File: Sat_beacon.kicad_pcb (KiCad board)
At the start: 2 copper layers, 79.5 x 122.9 mm, 126 parts, among them IC1 LMX2581ESQE_NOPB, IC2 LMX2581ESQE_NOPB, J1 Conn_01x05_Pin, J2 Conn_01x03_Pin, J4 MMCX, J5 MMCX, J6 Conn_01x04_Pin, Q1 BC817-40, Q2 BC817-40, Q3 BC817-40, Q4 BC817-40, SW1 B1407, SW2 SW_Omron_B3FS, SW3 SW_Omron_B3FS, SW4 SW_Omron_B3FS, SW5 SW_Omron_B3FS, U1 LD1117DT33, U2 LD1117DT33, U3 LD1117DT33, U4 1720BL15B0050002E, U5 1720BL15B0050002E, U7 STM32C031C6Tx, Y1 FT2MHUPM10.0-T1

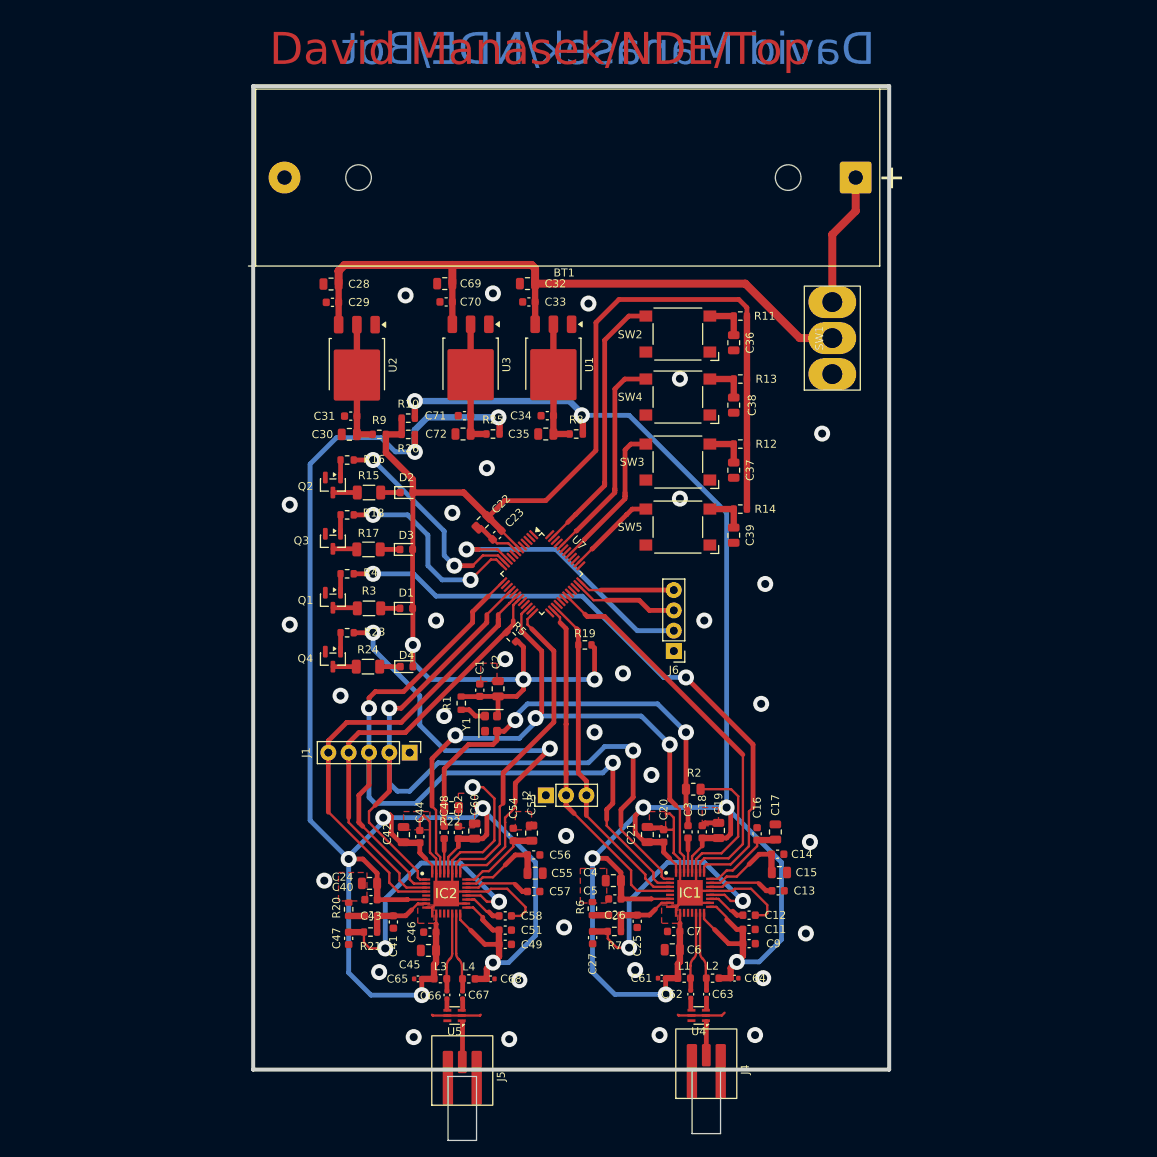
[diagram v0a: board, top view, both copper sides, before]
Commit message: PCB RF section improvement
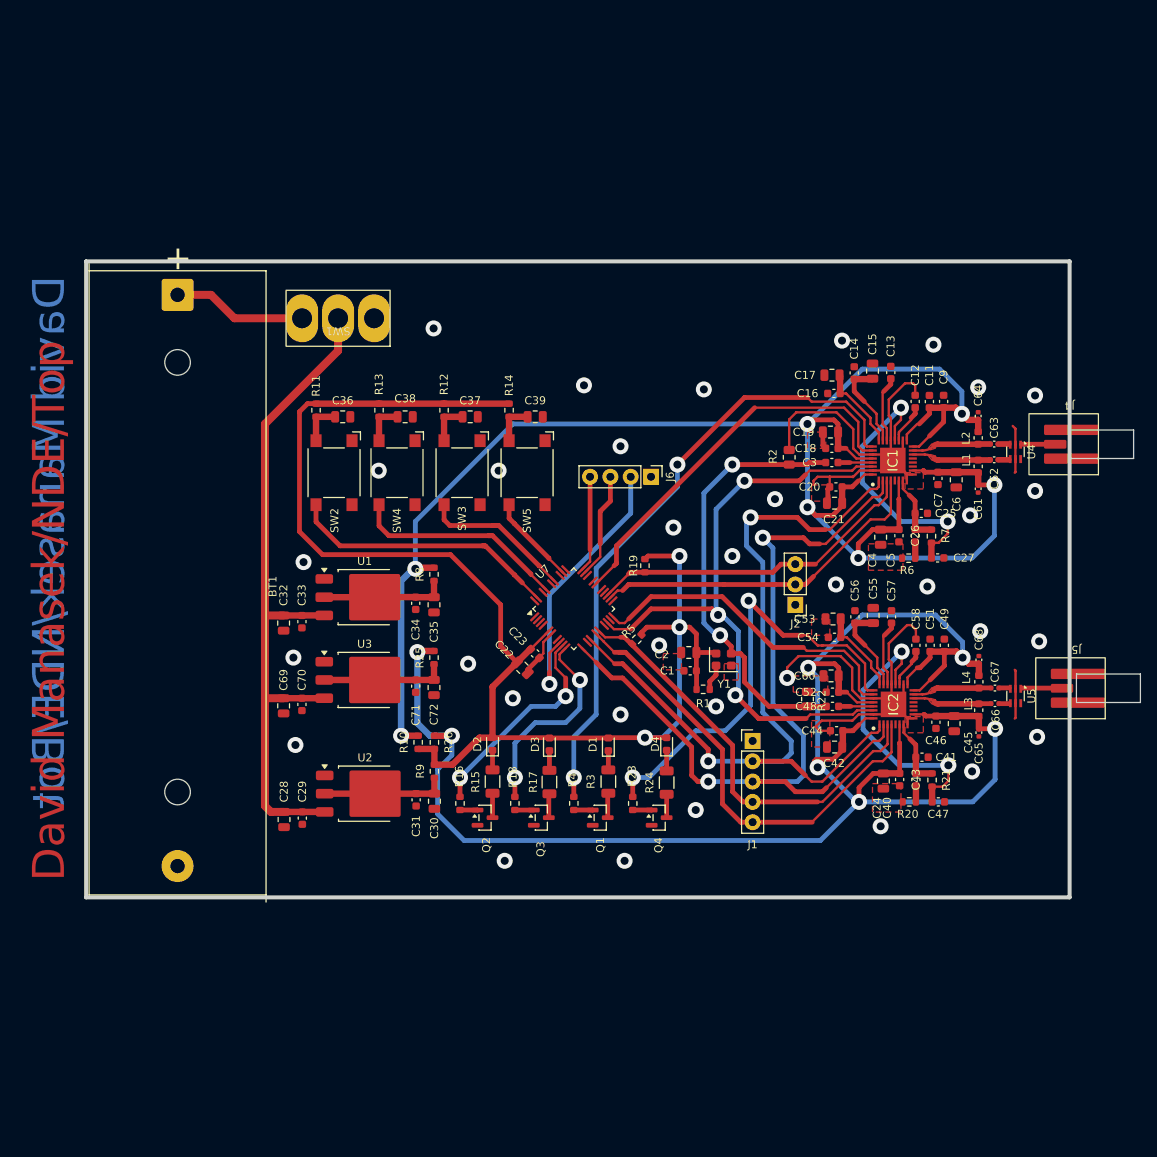
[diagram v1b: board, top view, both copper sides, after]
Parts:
- moved J5 90.8 mm to (169.2, 104.7), turned to 180 degrees
- moved J4 90.4 mm to (168.3, 74.2), turned to 180 degrees
- moved BT1 86.0 mm to (56.8, 55.6), turned to -90 degrees
- moved U4 80.8 mm to (161.6, 75.2), turned to -90 degrees
- moved U5 80.7 mm to (161.6, 105.7), turned to -90 degrees
- moved C63 77.6 mm to (158.9, 74.2), turned to 0 degrees
- moved C66 77.6 mm to (159.0, 106.7), turned to 0 degrees
- moved C67 76.8 mm to (159.0, 104.7), turned to 0 degrees
- moved C62 76.8 mm to (158.9, 76.2), turned to 0 degrees
- moved C64 76.6 mm to (156.9, 70.7), turned to 90 degrees
- moved C65 76.6 mm to (157.0, 110.3), turned to -90 degrees
- moved C47 75.7 mm to (151.9, 118.9), turned to 180 degrees
- moved L2 75.2 mm to (156.9, 73.4), turned to -90 degrees
- moved L3 75.2 mm to (157.0, 107.5), turned to -90 degrees
- moved L4 73.8 mm to (157.0, 103.9), turned to -90 degrees
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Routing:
- net /RF1_DC_N: track 9.93 -> 11.4 mm
- net /RF1_DC_P: track 9.94 -> 11.4 mm
- net /RF1_N: track 1.33 -> 2.70 mm
- net /RF1_P: track 1.30 -> 2.65 mm
- net Net-(SW1-B): track 86.1 -> 87.4 mm
- net VCC_PLL1: track 226.7 -> 227.2 mm
- added copper zone on F.Cu, net /RF1_DC_N
- added copper zone on F.Cu, net /RF1_DC_P
- added copper zone on F.Cu, net /RF2_DC_N
- added copper zone on F.Cu, net /RF2_DC_P
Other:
- board size 79.5 x 122.9 mm -> 122.9 x 79.5 mm
